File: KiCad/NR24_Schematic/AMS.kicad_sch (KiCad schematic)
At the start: 4 parts

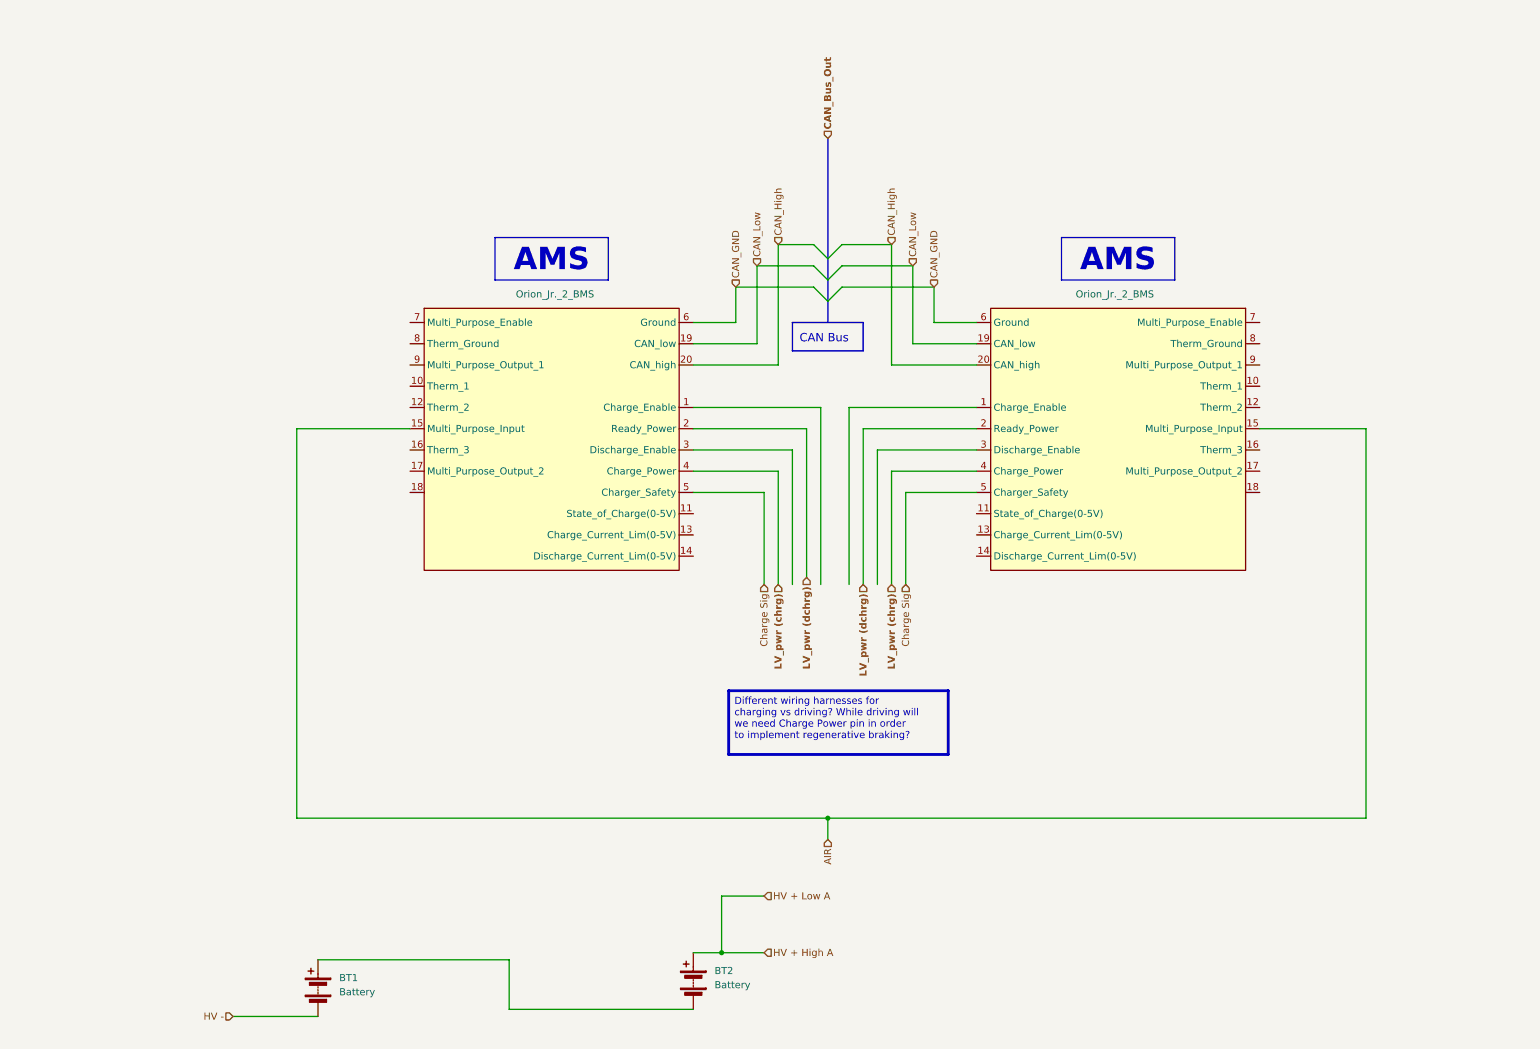
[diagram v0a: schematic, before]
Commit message: NOV1 Changes w Clarks
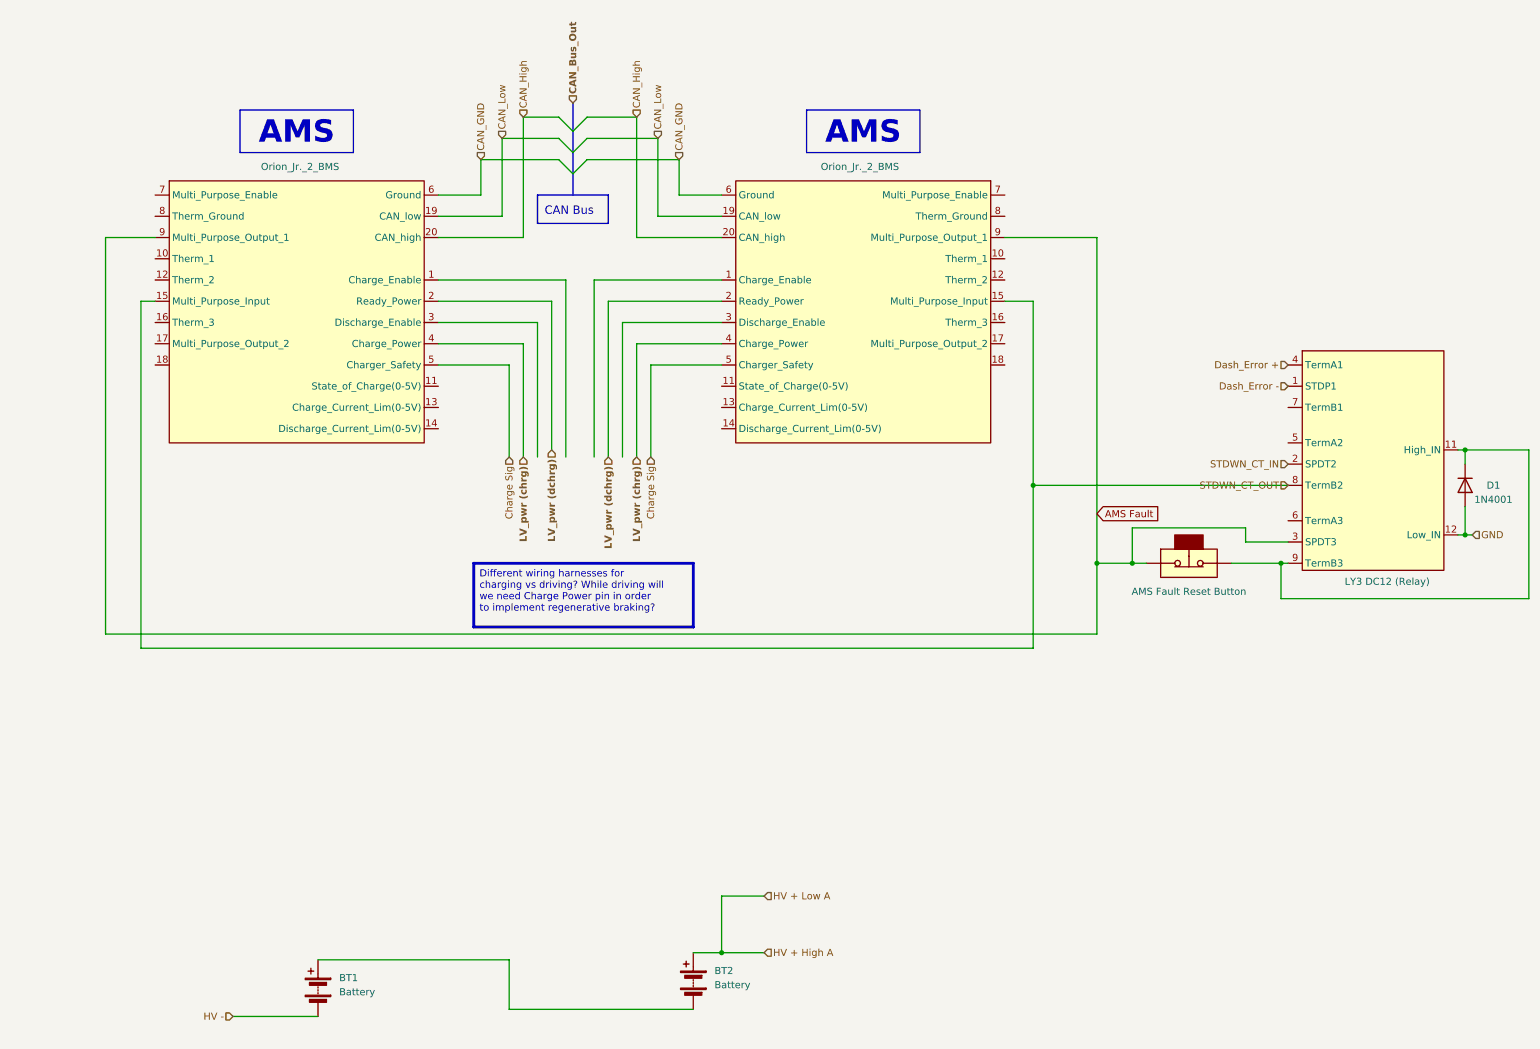
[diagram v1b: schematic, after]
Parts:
- added D1: 1N4001, Diode_THT:D_DO-41_SOD81_P10.16mm_Horizontal, symbol Diode:1N4001
- added SW?: AMS Fault Reset Button, symbol CamachosSymbols:Safety Switch
- added U?: LY3 DC12 (Relay), symbol CamachosSymbols:Sevcon_Gen4_Size6
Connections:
- net AMS Fault: now reaches U?.9 (Multi_Purpose_Output_1)
- net AMS Fault: now also U?.9 (Multi_Purpose_Output_1), SW?.1 (A), U?.3 (SPDT3)
- net AIR renamed STDWN_CT_OUT
- net STDWN_CT_OUT: now also U?.8 (TermB2)
- new net: D1.1 (K), SW?.2 (B), U?.11 (High_IN), U?.9 (TermB3)
- new net Dash_Error +: U?.4 (TermA1)
- new net Dash_Error -: U?.1 (STDP1)
- new net GND: D1.2 (A), U?.12 (Low_IN)
- new net STDWN_CT_IN: U?.2 (SPDT2)

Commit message: ams with IMD inside
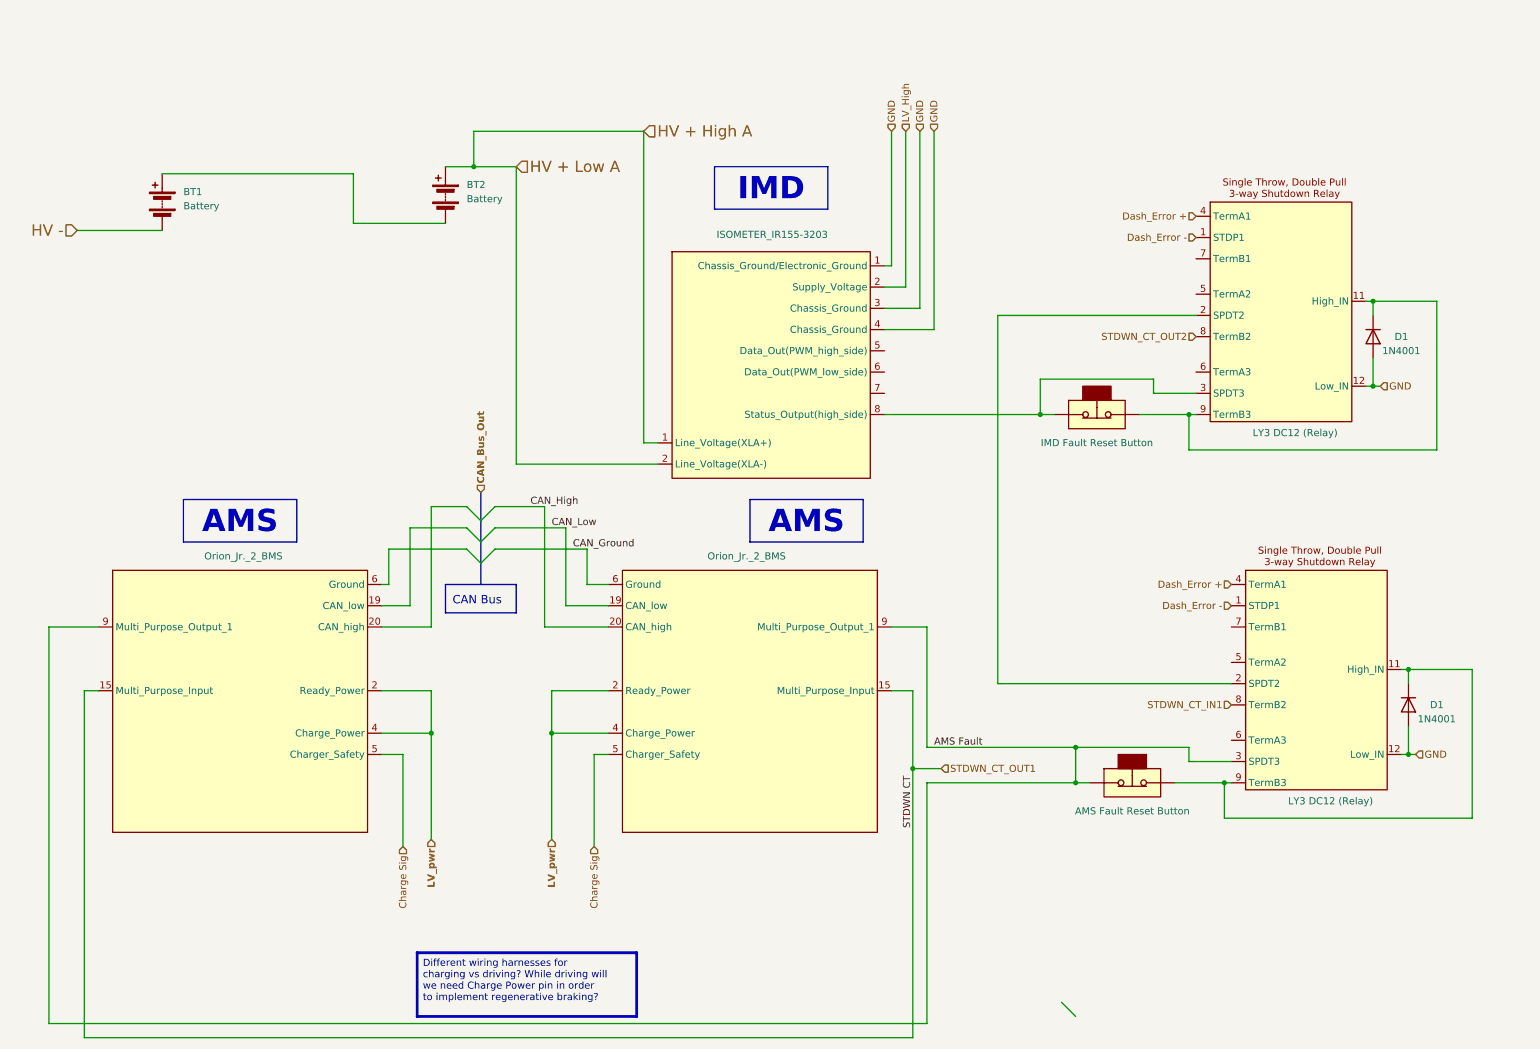
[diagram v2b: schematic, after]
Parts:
- removed U?: Orion_Jr._2_BMS, symbol CamachosSymbols:Sevcon_Gen4_Size6
- added D1: 1N4001, Diode_THT:D_DO-41_SOD81_P10.16mm_Horizontal, symbol Diode:1N4001
- added SW?: IMD Fault Reset Button, symbol CamachosSymbols:Safety Switch
- added U?: ISOMETER_IR155-3203, symbol CamachosSymbols:Sevcon_Gen4_Size6
- added U?: LY3 DC12 (Relay), symbol CamachosSymbols:Sevcon_Gen4_Size6
- added U?: Orion_Jr._2_BMS, symbol CamachosSymbols:Sevcon_Gen4_Size6
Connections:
- net LV_pwr (dchrg) is gone; now on net LV_pwr: U?.2 (Ready_Power)
- net AMS Fault: now also U?.9 (Multi_Purpose_Output_1)
- net Charge Sig: now also U?.5 (Charger_Safety)
- net Dash_Error +: now also U?.4 (TermA1)
- net Dash_Error -: now also U?.1 (STDP1)
- net GND: now also D1.2 (A), U?.1 (Line_Voltage(XLA+)), U?.12 (Low_IN), U?.3 (Chassis_Ground), U?.4 (Chassis_Ground)
- net HV + High A: now also U?.1 (Line_Voltage(XLA+)), U?.2 (Supply_Voltage)
- net CAN_GND renamed CAN_Ground
- net LV_pwr (chrg) renamed LV_pwr
- net LV_pwr: now also U?.2 (Ready_Power), U?.4 (Charge_Power)
- net STDWN_CT_IN: no longer names the net of U?.2 (SPDT2)
- net STDWN_CT_IN: now also U?.2 (SPDT2)
- net STDWN_CT_OUT renamed STDWN_CT_IN1
- net STDWN_CT_IN1: no longer U?.15 (Multi_Purpose_Input)
- new net: SW?.1 (A), U?.3 (SPDT3), U?.8 (Status_Output(high_side))
- new net: D1.1 (K), SW?.2 (B), U?.11 (High_IN), U?.9 (TermB3)
- new net LV_High: U?.2 (Supply_Voltage)
- new net STDWN_CT_OUT1: U?.15 (Multi_Purpose_Input), U?.15 (Multi_Purpose_Input)
- new net STDWN_CT_OUT2: U?.8 (TermB2)
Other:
- moved on the sheet: BT1, BT2, D1
